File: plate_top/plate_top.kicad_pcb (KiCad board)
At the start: 2 copper layers, 174.6 x 118.1 mm, 35 parts, among them J1 TRRS, J3 OLED, SW1 SW_Push, SW20 SW_Push, SW27 SW_Push, SW28 SW_Push, SW29 SW_Push, SW30 SW_Push, SW31 SW_Push, SW32 SW_Push, U1 ProMicro

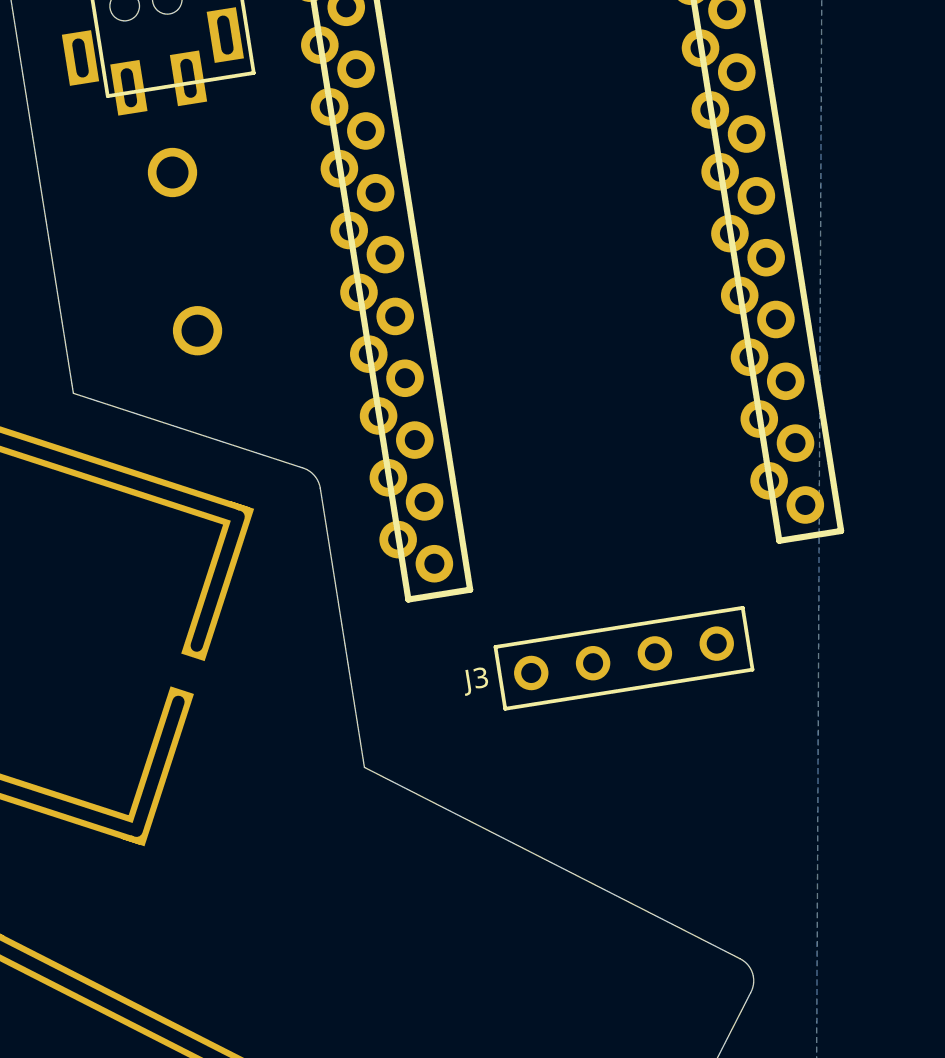
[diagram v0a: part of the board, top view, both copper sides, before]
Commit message: Multiple fixes...
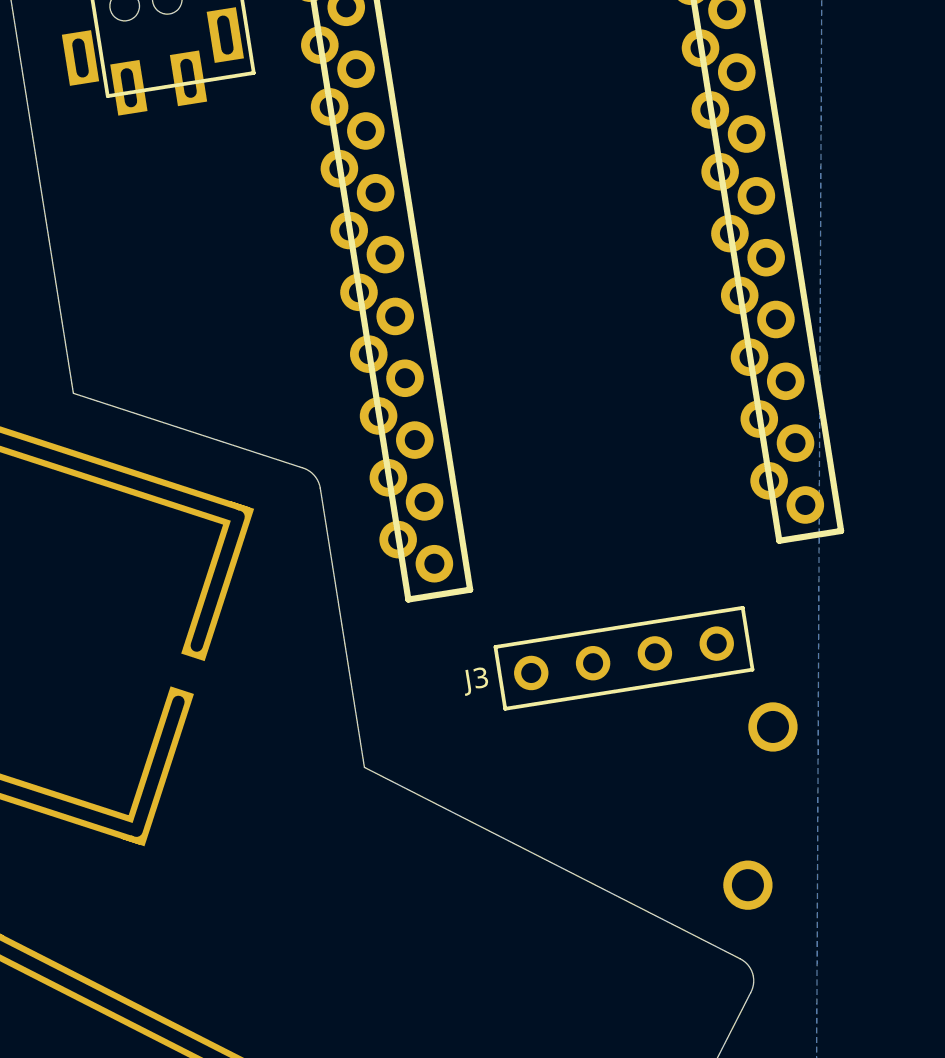
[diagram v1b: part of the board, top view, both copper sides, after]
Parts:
- moved SW32 32.4 mm to (251.4, 98.1), turned to 81 degrees
